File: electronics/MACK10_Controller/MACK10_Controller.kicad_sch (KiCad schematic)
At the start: 0 parts

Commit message: Added KiCad and Electronics Files
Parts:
- added M1: Stepper_Motor_bipolar, symbol Motor:Stepper_Motor_bipolar
- added U1: U1 ESP32_DEVKIT_30P, MACK10:ESP32_DEVKIT_30PIN, symbol MACK10:ESP32_DEVKIT_30P
- added U2: HX711, MACK10:HX711_MODULE, symbol MACK10:HX711_MODULE
- added U3: TMC2208, MACK10:TMC2208_STEPSTICK, symbol MACK10:TMC2208_STEPSTICK
- added U4: LOAD CELL, symbol MACK10:LOAD_CELL_4P
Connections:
- new net: M1.1, U3.12 (1A)
- new net: M1.2 (-), U3.11 (1B)
- new net: M1.3, U3.13 (2A)
- new net: M1.4, U3.14 (2B)
- new net 3V3: U1.1 (3V3), U2.10 (VCC), U3.15 (VIO)
- new net DIR: U1.10 (D19), U3.8 (DIR)
- new net ENABLE: U1.8 (D5), U3.1 (EN)
- new net GND: U1.2 (GND), U2.7 (GND), U3.10 (GND), U3.16 (GND)
- new net HX711_DT: U1.11 (D21), U2.8 (DT)
- new net HX711_SCK: U1.14 (D22), U2.9 (SCK)
- new net LOAD_A+: U2.3 (A-), U4.3 (Pin_3)
- new net LOAD_A-: U2.4 (A+), U4.4 (Pin_4)
- new net LOAD_E+: U2.1 (E+), U4.1 (Pin_1)
- new net LOAD_E-: U2.2 (E-), U4.2 (Pin_2)
- new net STEP: U1.9 (D18), U3.7 (STEP)
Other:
- title: (none) -> MACK-10 Controller

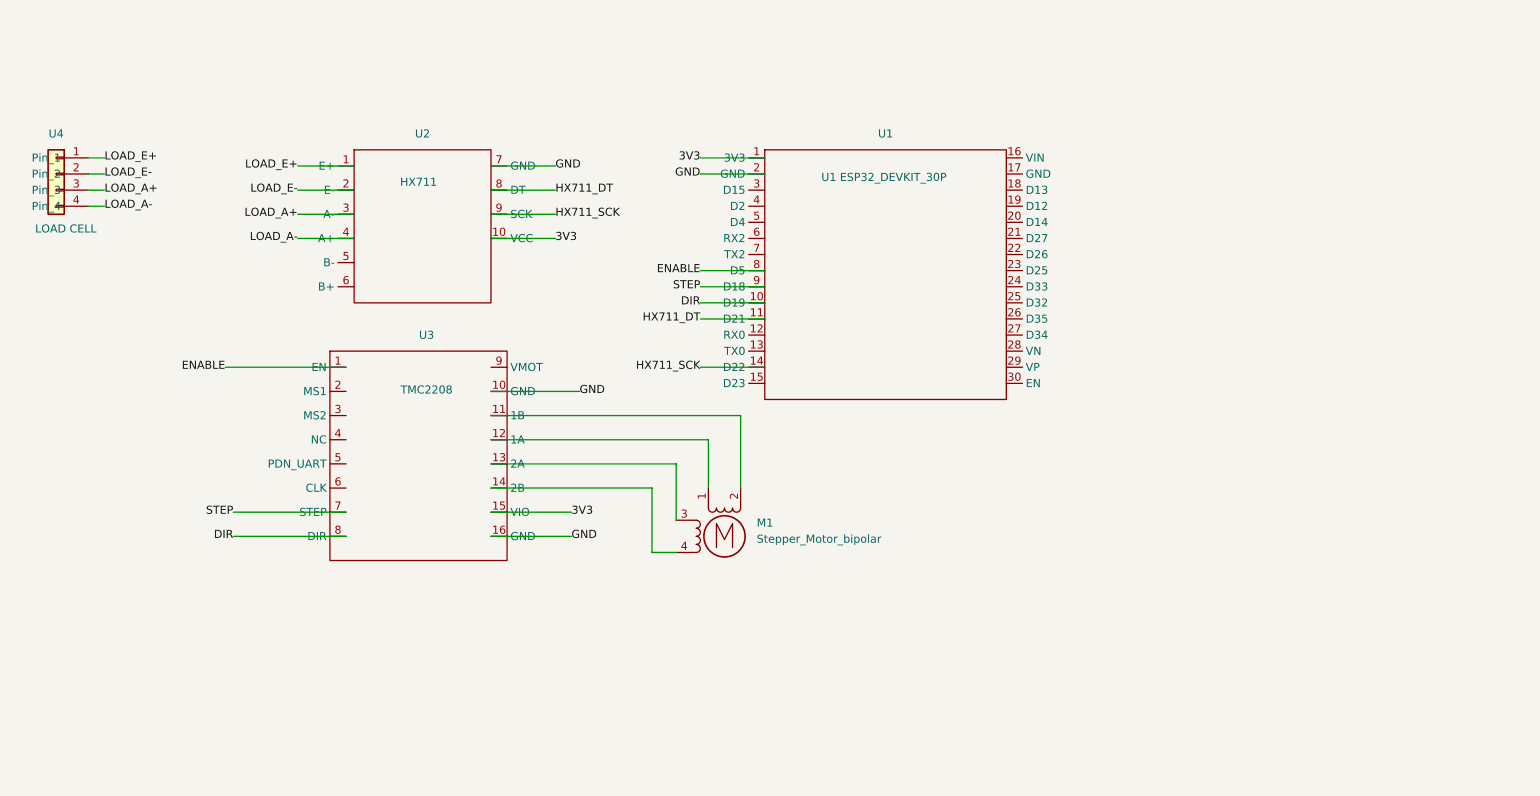
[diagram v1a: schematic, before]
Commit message: Initial PCB Layout
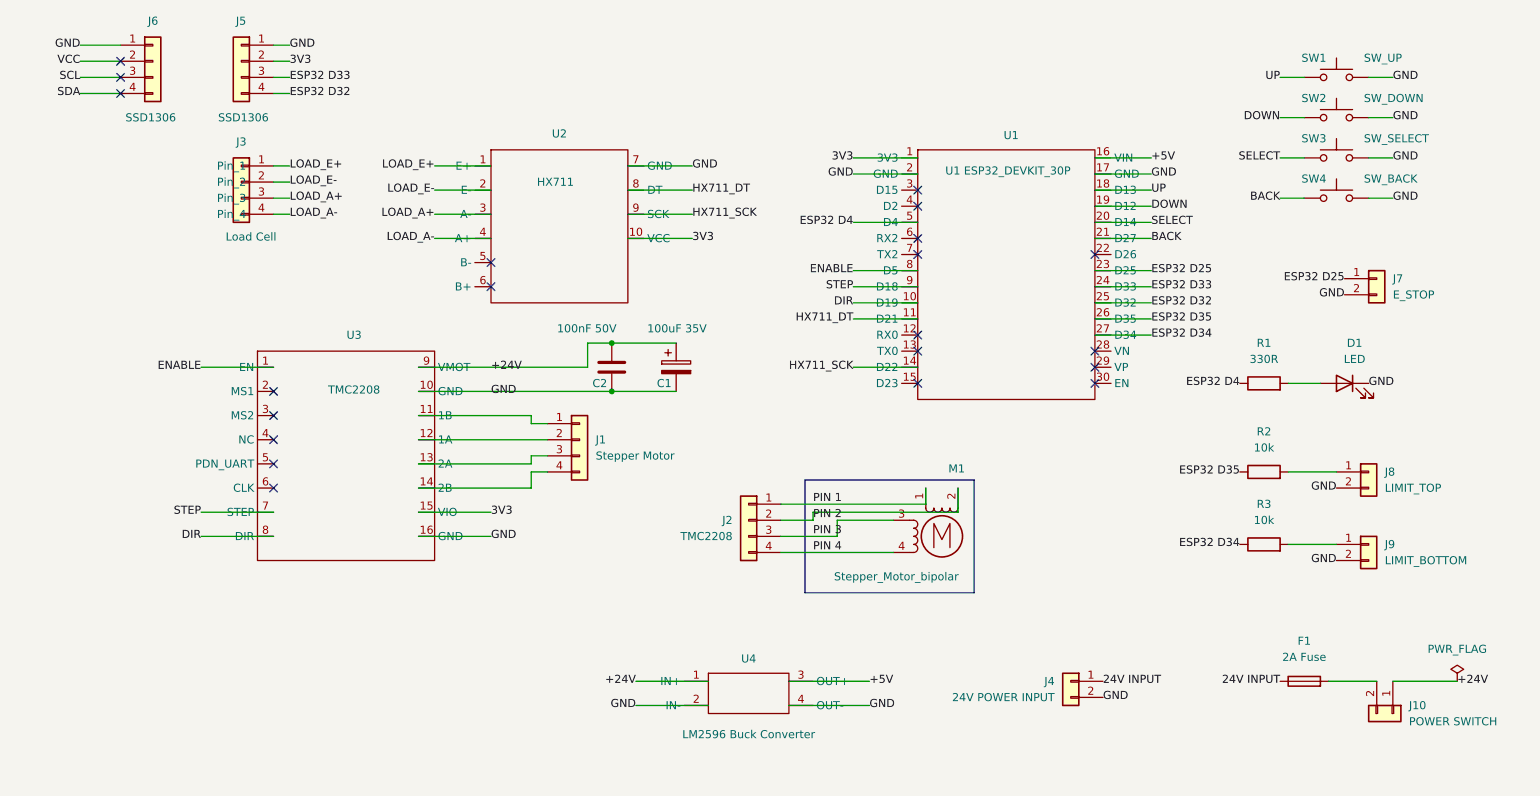
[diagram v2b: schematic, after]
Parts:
- added C1: 100uF 35V, Capacitor_THT:CP_Radial_D8.0mm_P3.50mm, symbol Device:C_Polarized
- added C2: 100nF 50V, Capacitor_THT:C_Disc_D5.0mm_W2.5mm_P5.00mm, symbol Device:C
- added D1: LED, LED_THT:LED_D5.0mm, symbol Device:LED
- added F1: 2A Fuse, Fuse:Fuseholder_Blade_Mini_Keystone_3568, symbol Device:Fuse
- added J1: Stepper Motor, Connector_PinHeader_2.54mm:PinHeader_1x04_P2.54mm_Vertical, symbol Connector_Generic:Conn_01x04
- added J10: POWER SWITCH, Connector_PinHeader_2.54mm:PinHeader_1x02_P2.54mm_Vertical, symbol Connector_Generic:Conn_01x02
- added J2: TMC2208, Connector_PinHeader_2.54mm:PinHeader_1x04_P2.54mm_Vertical, symbol Connector_Generic:Conn_01x04
- added J4: 24V POWER INPUT, Connector_PinHeader_2.54mm:PinHeader_1x04_P2.54mm_Vertical, symbol Connector_Generic:Conn_01x02
- added J5, J6: SSD1306, Connector_PinHeader_2.54mm:PinHeader_1x04_P2.54mm_Vertical, symbol Connector_Generic:Conn_01x04
- added J7: E_STOP, Connector_PinHeader_2.54mm:PinHeader_1x04_P2.54mm_Vertical, symbol Connector_Generic:Conn_01x02
- added J8: LIMIT_TOP, Connector_PinHeader_2.54mm:PinHeader_1x04_P2.54mm_Vertical, symbol Connector_Generic:Conn_01x02
- added J9: LIMIT_BOTTOM, Connector_PinHeader_2.54mm:PinHeader_1x04_P2.54mm_Vertical, symbol Connector_Generic:Conn_01x02
- added R1: 330R, Resistor_THT:R_Axial_DIN0207_L6.3mm_D2.5mm_P10.16mm_Horizontal, symbol Device:R
- added R2, R3: 10k, Resistor_THT:R_Axial_DIN0207_L6.3mm_D2.5mm_P10.16mm_Horizontal, symbol Device:R
- added SW1: SW_UP, Button_Switch_THT:SW_PUSH_6mm, symbol Switch:SW_Push
- added SW2: SW_DOWN, Button_Switch_THT:SW_PUSH_6mm, symbol Switch:SW_Push
- added SW3: SW_SELECT, Button_Switch_THT:SW_PUSH_6mm, symbol Switch:SW_Push
- added SW4: SW_BACK, Button_Switch_THT:SW_PUSH_6mm, symbol Switch:SW_Push
- added U4: LM2596 Buck Converter, MACK10:LM2596_BUCK_CONVERTER, symbol MACK10:LM2596_MODULE
- J3: renamed from U4; value LOAD CELL -> Load Cell; footprint (none) -> Connector_PinHeader_2.54mm:PinHeader_1x04_P2.54mm_Vertical
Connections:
- net 3V3: now also J5.2 (Pin_2)
- net GND: now also U1.17 (GND), C1.2, C2.2, D1.1 (K), J4.2 (Pin_2), J5.1 (Pin_1), J6.1 (Pin_1), J7.2 (Pin_2), J8.2 (Pin_2), J9.2 (Pin_2), SW1.2, SW2.2, SW3.2, SW4.2, U4.2 (IN-), U4.4 (OUT-)
- net +5V: now reaches U1.16 (VIN)
- net +5V: now also U4.3 (OUT+)
- net UP: now reaches U1.18 (D13)
- net UP: now also SW1.1
- net DOWN: now reaches U1.19 (D12)
- net DOWN: now also SW2.1
- net SELECT: now reaches U1.20 (D14)
- net SELECT: now also SW3.1
- net BACK: now reaches U1.21 (D27)
- net BACK: now also SW4.1
- net ESP32 D25: now reaches U1.23 (D25)
- net ESP32 D25: now also J7.1 (Pin_1)
- net ESP32 D33: now reaches U1.24 (D33)
- net ESP32 D33: now also J5.3 (Pin_3)
- net ESP32 D32: now reaches U1.25 (D32)
- net ESP32 D32: now also J5.4 (Pin_4)
- net ESP32 D35: now reaches U1.26 (D35)
- net ESP32 D35: now also R2.1
- net ESP32 D34: now reaches U1.27 (D34)
- net ESP32 D34: now also R3.1
- net ESP32 D4: now reaches U1.5 (D4)
- net ESP32 D4: now also R1.1
- net at U3.12 (1A): now also J1.2 (Pin_2); no longer M1.1
- net at U3.11 (1B): now also J1.1 (Pin_1); no longer M1.2 (-)
- net at U3.13 (2A): now also J1.3 (Pin_3); no longer M1.3
- net at U3.14 (2B): now also J1.4 (Pin_4); no longer M1.4
- net +24V: now reaches U3.9 (VMOT)
- net +24V: now also C1.1, C2.1, J10.1 (Pin_1), U4.1 (IN+)
- new net: J8.1 (Pin_1), R2.2
- new net: F1.2, J10.2 (Pin_2)
- new net: J9.1 (Pin_1), R3.2
- new net: D1.2 (A), R1.2
- new net 24V INPUT: F1.1, J4.1 (Pin_1)
- new net PIN 1: J2.1 (Pin_1), M1.1
- new net PIN 2: J2.2 (Pin_2), M1.2 (-)
- new net PIN 3: J2.3 (Pin_3), M1.3
- new net PIN 4: J2.4 (Pin_4), M1.4
- new net SCL: J6.3 (Pin_3)
- new net SDA: J6.4 (Pin_4)
- new net VCC: J6.2 (Pin_2)
- no-connect marks 0 -> 21
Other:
- moved on the sheet: J3, M1, U1, U2, U3

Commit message: Update PCB Layout
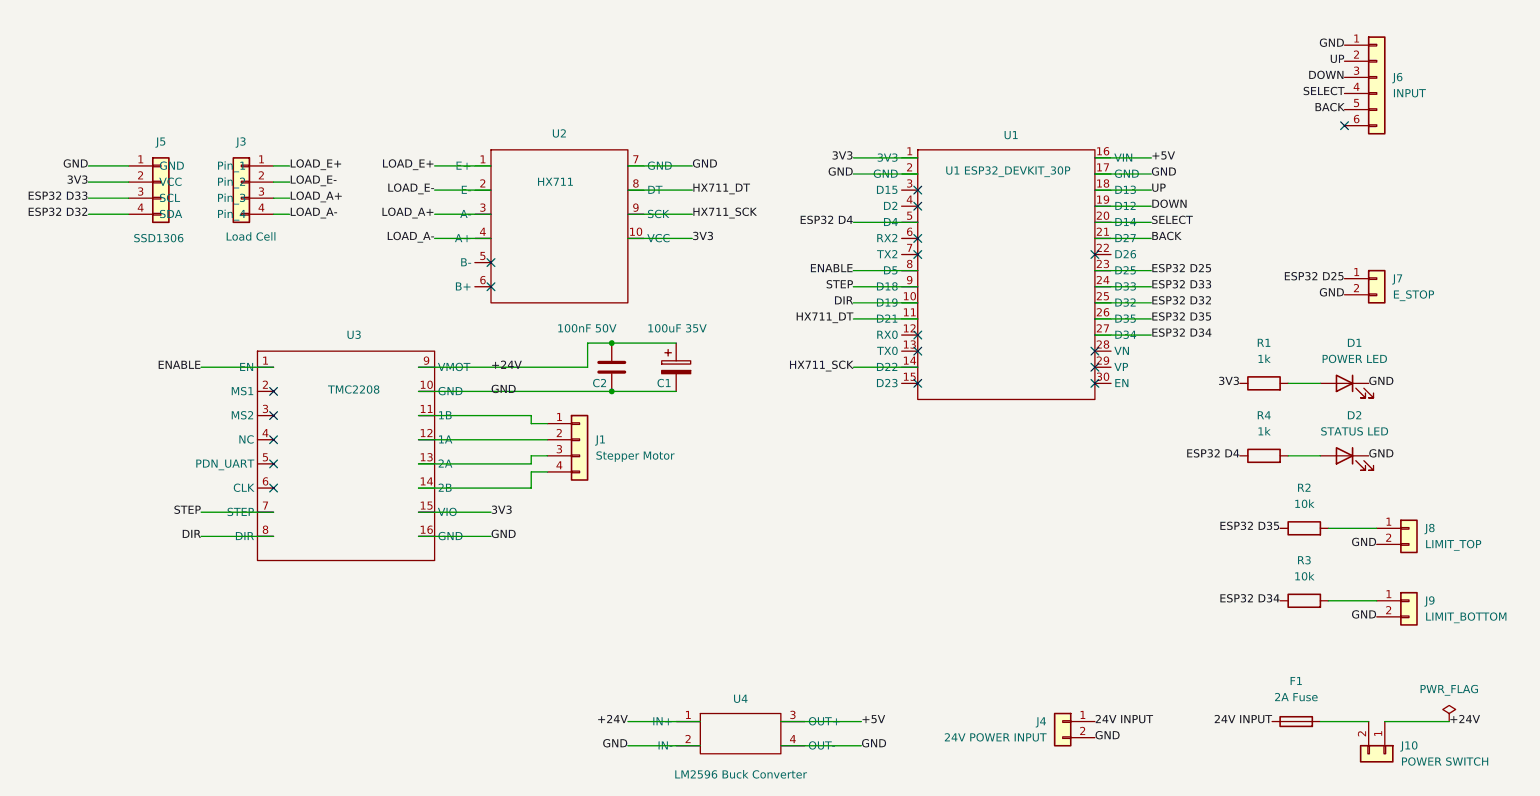
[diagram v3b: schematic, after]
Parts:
- removed J2: TMC2208, Connector_PinHeader_2.54mm:PinHeader_1x04_P2.54mm_Vertical, symbol Connector_Generic:Conn_01x04
- removed J5: SSD1306, Connector_PinHeader_2.54mm:PinHeader_1x04_P2.54mm_Vertical, symbol Connector_Generic:Conn_01x04
- removed M1: Stepper_Motor_bipolar, symbol Motor:Stepper_Motor_bipolar
- removed SW1: SW_UP, Button_Switch_THT:SW_PUSH_6mm, symbol Switch:SW_Push
- removed SW2: SW_DOWN, Button_Switch_THT:SW_PUSH_6mm, symbol Switch:SW_Push
- removed SW3: SW_SELECT, Button_Switch_THT:SW_PUSH_6mm, symbol Switch:SW_Push
- removed SW4: SW_BACK, Button_Switch_THT:SW_PUSH_6mm, symbol Switch:SW_Push
- added D2: STATUS LED, LED_SMD:LED_0805_2012Metric_Pad1.15x1.40mm_HandSolder, symbol Device:LED
- added J6: INPUT, Connector_JST:JST_XH_B6B-XH-A_1x06_P2.50mm_Vertical, symbol Connector_Generic:Conn_01x06
- added R4: 1k, Resistor_THT:R_Axial_DIN0207_L6.3mm_D2.5mm_P10.16mm_Horizontal, symbol Device:R
- D1: value LED -> POWER LED; footprint LED_THT:LED_D5.0mm -> LED_SMD:LED_0805_2012Metric_Pad1.15x1.40mm_HandSolder
- J1, J3: footprint Connector_PinHeader_2.54mm:PinHeader_1x04_P2.54mm_Vertical -> Connector_JST:JST_XH_B4B-XH-A_1x04_P2.50mm_Vertical
- J4, J7, J8, J9: footprint Connector_PinHeader_2.54mm:PinHeader_1x04_P2.54mm_Vertical -> Connector_JST:JST_XH_B2B-XH-A_1x02_P2.50mm_Vertical
- J5: renamed from J6; footprint Connector_PinHeader_2.54mm:PinHeader_1x04_P2.54mm_Vertical -> Connector_JST:JST_XH_B4B-XH-A_1x04_P2.50mm_Vertical
- R1: value 330R -> 1k
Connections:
- net SCL is gone; now on net ESP32 D33: J5.3 (SCL)
- net SDA is gone; now on net ESP32 D32: J5.4 (SDA)
- net VCC is gone; now on net 3V3: J5.2 (VCC)
- net 3V3: now also R1.1
- net BACK: now also J6.5 (Pin_5)
- net DOWN: now also J6.3 (Pin_3)
- net ESP32 D4: now also R4.1; no longer R1.1
- net GND: now also D2.1 (K), J6.1 (Pin_1)
- net SELECT: now also J6.4 (Pin_4)
- net UP: now also J6.2 (Pin_2)
- new net: D2.2 (A), R4.2
- no-connect marks 21 -> 19
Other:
- moved on the sheet: F1, J10, J4, J8, J9, R2, R3, U4
